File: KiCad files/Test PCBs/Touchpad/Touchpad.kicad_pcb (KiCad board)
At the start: 2 copper layers, 78.3 x 50.7 mm, 35 parts, among them J1 Conn_02x03_Counter_Clockwise, J2 Conn_02x03_Counter_Clockwise, J3 Conn_01x07_Male, U1 TTP223-BA6, U2 TTP223-BA6, U3 TTP223-BA6

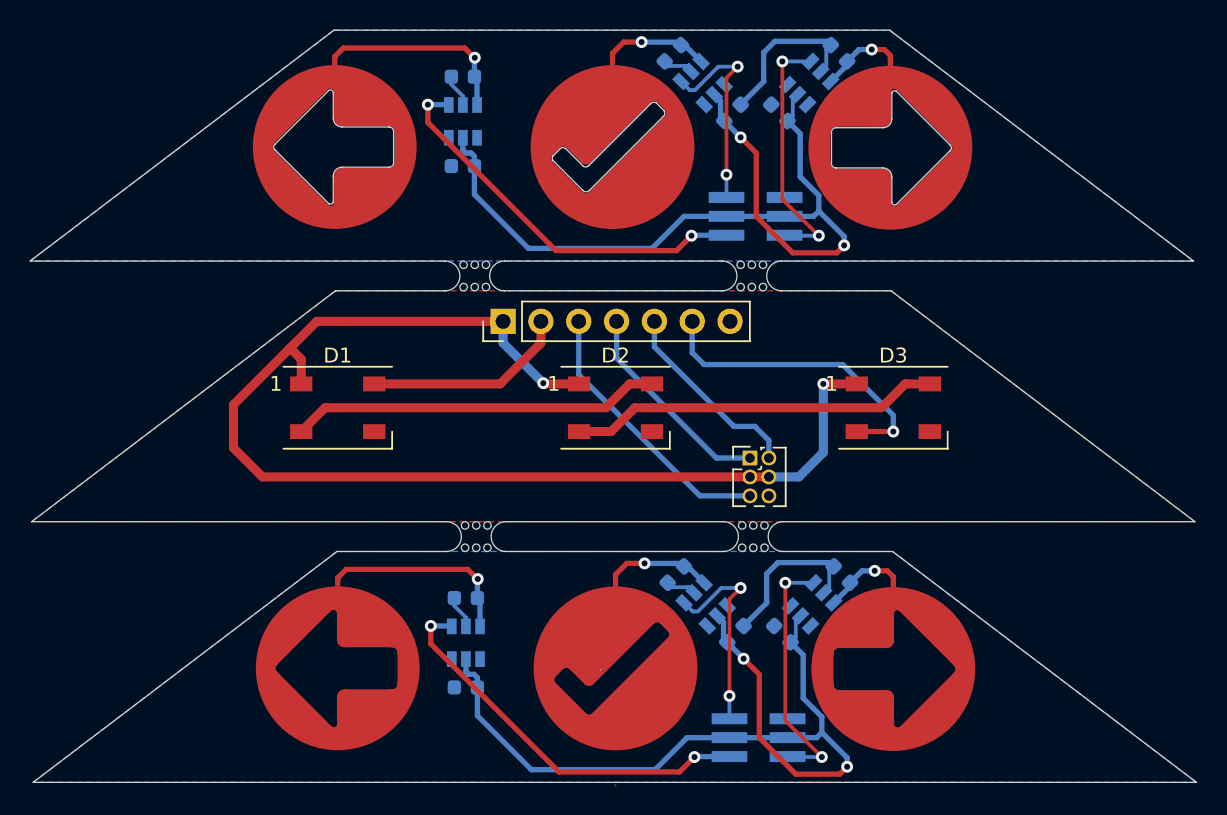
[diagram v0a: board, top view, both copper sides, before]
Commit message: update
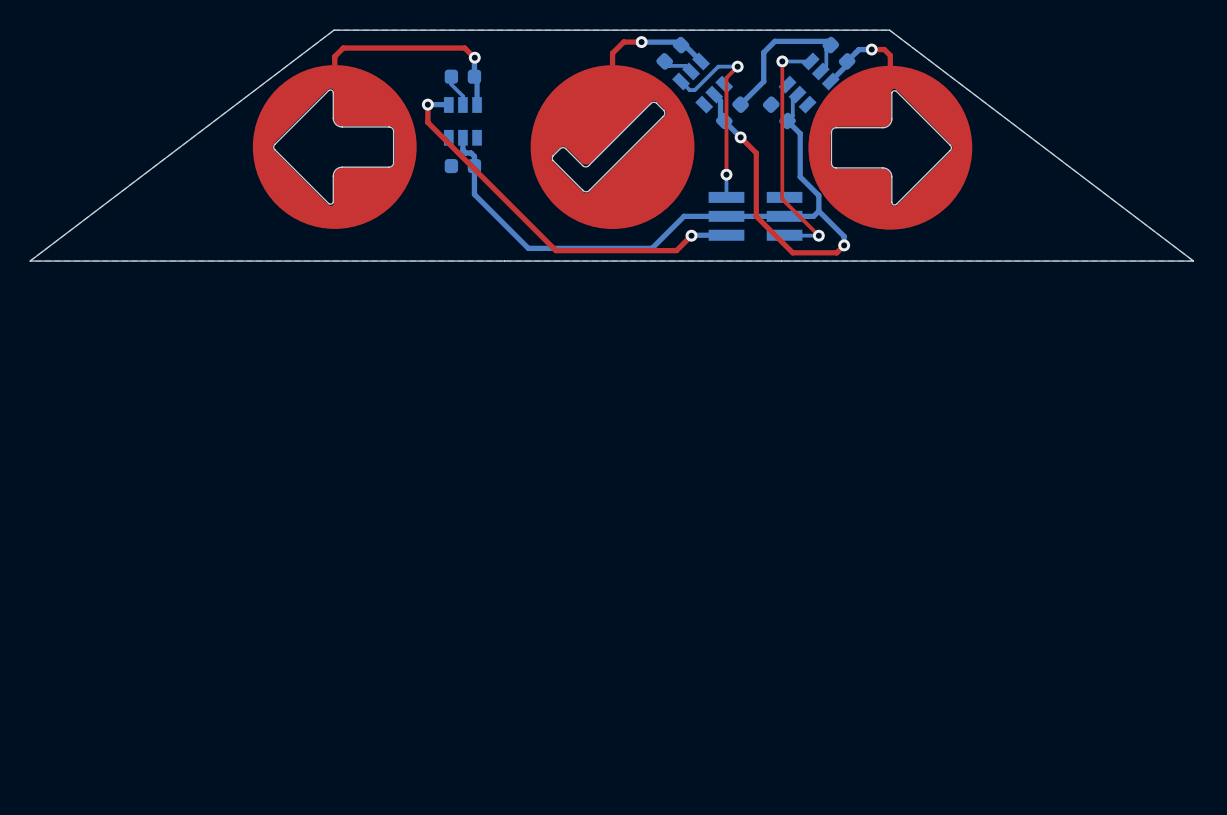
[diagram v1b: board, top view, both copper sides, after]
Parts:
- removed the C1 at (202.9, 100.2)
- removed the C2 at (206.9, 104.2)
- removed the C3 at (188.9, 101.8)
- removed the C4 at (188.9, 107.8)
- removed the C5 at (214.1, 100.2)
- removed the C6 at (210.1, 104.2)
- removed D1, D2, D3: WS2812B, LED_SMD:LED_WS2812B_PLCC4_5.0x5.0mm_P3.2mm
- removed the J1 at (208.5, 111.2)
- removed J2: Conn_02x03_Counter_Clockwise, Connector_PinHeader_1.27mm:PinHeader_2x03_P1.27mm_Vertical
- removed J3: Conn_01x07_Male, Connector_PinHeader_2.54mm:PinHeader_1x07_P2.54mm_Vertical
- removed the TP1 at (198.9, 106.5)
- removed the TP2 at (180.2, 106.5)
- removed the TP3 at (217.6, 106.5)
- removed the U1 at (204.9, 102.2)
- removed the U2 at (188.9, 104.8)
- removed the U3 at (212.1, 102.2)
- removed mouse-bite-2mm-slot (x4): VAL**, Touchpad:mouse-bite-2mm-slot
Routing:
- net +5V: track 199.2 -> 58.8 mm, vias 6 -> 2
- net TP2: track 67.5 -> 26.7 mm, vias 4 -> 2
- net TP1: track 46.0 -> 13.8 mm, vias 4 -> 2
- net TP3: track 47.0 -> 16.9 mm, vias 4 -> 2
- net Net-(D2-Pad2): track 24.9 -> 0.00 mm
- net Net-(D1-Pad2): track 24.9 -> 0.00 mm
- net Net-(D3-Pad2): track 20.9 -> 0.00 mm, vias 1 -> 0
- net GND: track 30.8 -> 15.4 mm
- net Net-(D1-Pad4): track 13.8 -> 0.00 mm
- net Net-(C3-Pad1): track 26.6 -> 13.3 mm, vias 2 -> 1
- net Net-(C1-Pad1): track 14.2 -> 7.10 mm, vias 2 -> 1
- net Net-(C5-Pad1): track 10.8 -> 5.40 mm, vias 2 -> 1
- removed copper zone on F.Cu, net GND
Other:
- board size 78.3 x 50.7 mm -> 78.1 x 15.5 mm
- board text removed: "5V"
- board text removed: "GND"
- board text removed: "IN"
- board text removed: "OUT"
- board text removed: "TP1"
- board text removed: "TP2"
- board text removed: "TP3"

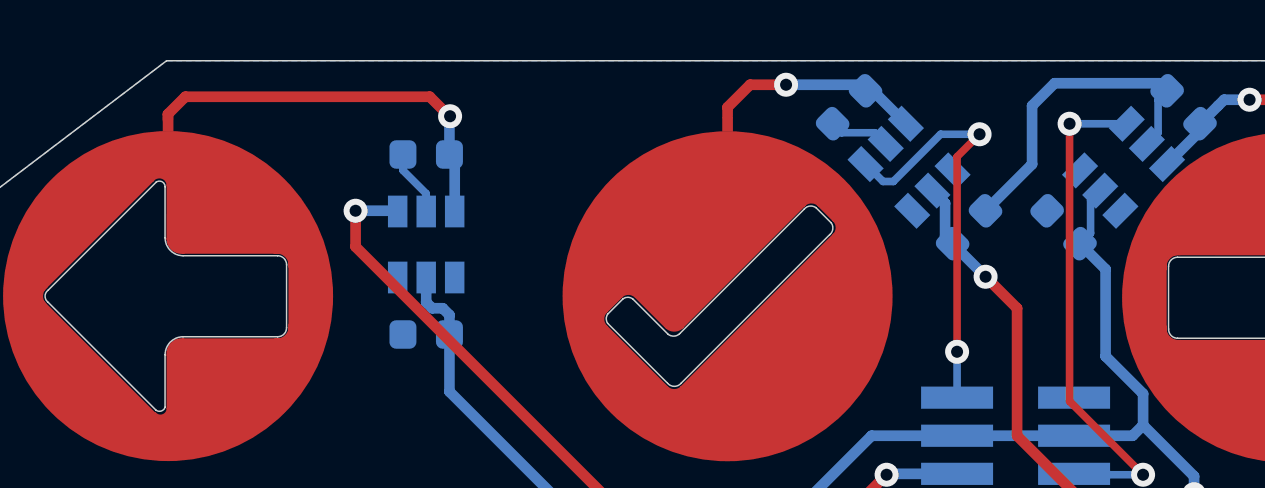
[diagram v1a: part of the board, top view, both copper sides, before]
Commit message: buzzer
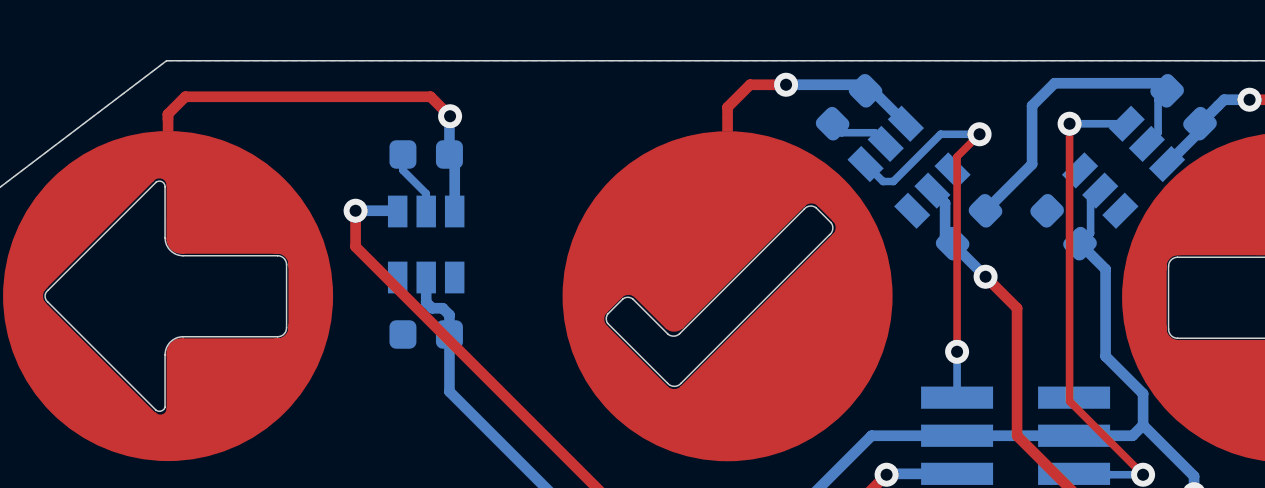
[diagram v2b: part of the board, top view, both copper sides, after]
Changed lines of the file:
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@@
   (segment (start 189.429045 72.775) (end 189.429045 72.125) (width 0.3556) (layer "B.Cu") (net 9))
   (segment (start 189.429045 72.125) (end 189.204045 71.9) (width 0.3556) (layer "B.Cu") (net 9))
-  (segment (start 210.448008 69.748008) (end 210.451992 69.748008) (width 0.254) (layer "B.Cu") (net 9))
-  (segment (start 210.448008 69.748008) (end 210.448008 69.701992) (width 0.254) (layer "B.Cu") (net 9))
   (segment (start 214.25 77.5) (end 212.55 75.8) (width 0.3556) (layer "B.Cu") (net 9))
   (segment (start 189.429045 72.775) (end 189.429045 74.679045) (width 0.3556) (layer "B.Cu") (net 9))
@@
   (segment (start 212.55 74.75) (end 211.3 73.5) (width 0.3556) (layer "B.Cu") (net 9))
   (segment (start 205.95 69.5) (end 205.95 68.4) (width 0.3556) (layer "B.Cu") (net 9))
-  (segment (start 210.25 69.946016) (end 210.448008 69.748008) (width 0.3556) (layer "B.Cu") (net 9))
   (segment (start 198.7 65.2) (end 198.7 65.5) (width 0.3556) (layer "F.Cu") (net 12))
   (segment (start 200.65 64.45) (end 199.45 64.45) (width 0.3556) (layer "F.Cu") (net 12))
@@
   (segment (start 203.298008 64.651992) (end 203.298008 64.648008) (width 0.254) (layer "B.Cu") (net 12))
   (segment (start 203.545495 64.651992) (end 204.643934 65.750431) (width 0.3556) (layer "B.Cu") (net 12))
-  (segment (start 188.775 64.85) (end 180.625 64.85) (width 0.3556) (layer "F.Cu") (net 13))
-  (segment (start 189.425 65.5) (end 188.775 64.85) (width 0.3556) (layer "F.Cu") (net 13))
+  (segment (start 180.625 64.85) (end 180.043597 65.431403) (width 0.3556) (layer "F.Cu") (net 13))
   (segment (start 180.043597 65.431403) (end 180.043597 65.613493) (width 0.3556) (layer "F.Cu") (net 13))
-  (segment (start 180.625 64.85) (end 180.043597 65.431403) (width 0.3556) (layer "F.Cu") (net 13))
+  (segment (start 189.45 65.5) (end 188.8 64.85) (width 0.3556) (layer "F.Cu") (net 13))
+  (segment (start 188.8 64.85) (end 180.625 64.85) (width 0.3556) (layer "F.Cu") (net 13))
   (via (at 189.45 65.5) (size 0.8) (drill 0.4) (layers "F.Cu" "B.Cu") (net 13))
   (segment (start 189.429045 65.504045) (end 189.425 65.5) (width 0.3556) (layer "B.Cu") (net 13))
+  (segment (start 189.429045 65.520955) (end 189.45 65.5) (width 0.3556) (layer "B.Cu") (net 13))
   (segment (start 189.604045 68.675) (end 189.604045 66.95) (width 0.3556) (layer "B.Cu") (net 13))
-  (segment (start 189.429045 66.775) (end 189.429045 65.504045) (width 0.3556) (layer "B.Cu") (net 13))
+  (segment (start 189.429045 66.775) (end 189.429045 65.520955) (width 0.3556) (layer "B.Cu") (net 13))
   (segment (start 189.604045 66.95) (end 189.429045 66.775) (width 0.3556) (layer "B.Cu") (net 13))
   (segment (start 206.35 73.35) (end 206.35 66.85) (width 0.254) (layer "F.Cu") (net 14))
